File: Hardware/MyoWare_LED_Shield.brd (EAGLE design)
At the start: 52.3 x 21.6 mm, 21 parts, among them IC1 LM3914V, U1 MCP73831

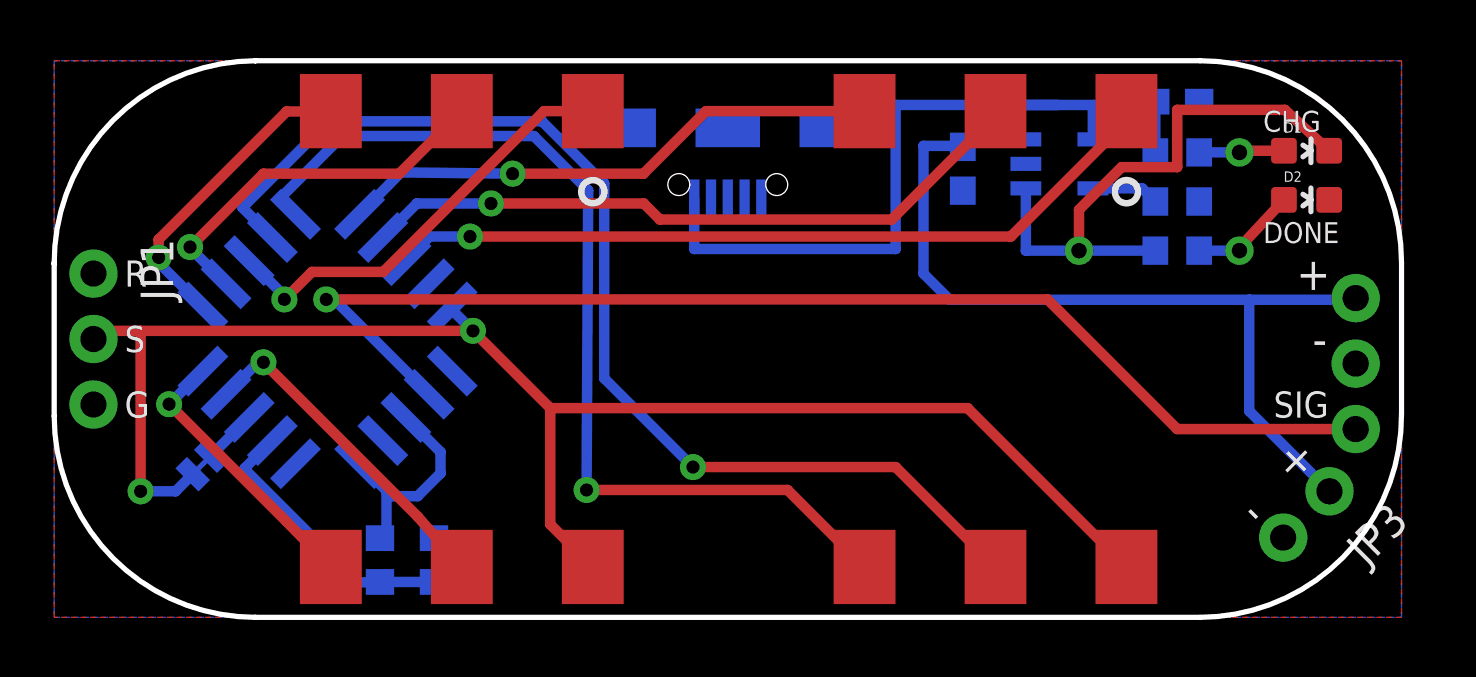
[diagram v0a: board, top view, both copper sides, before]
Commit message: Design rules checked
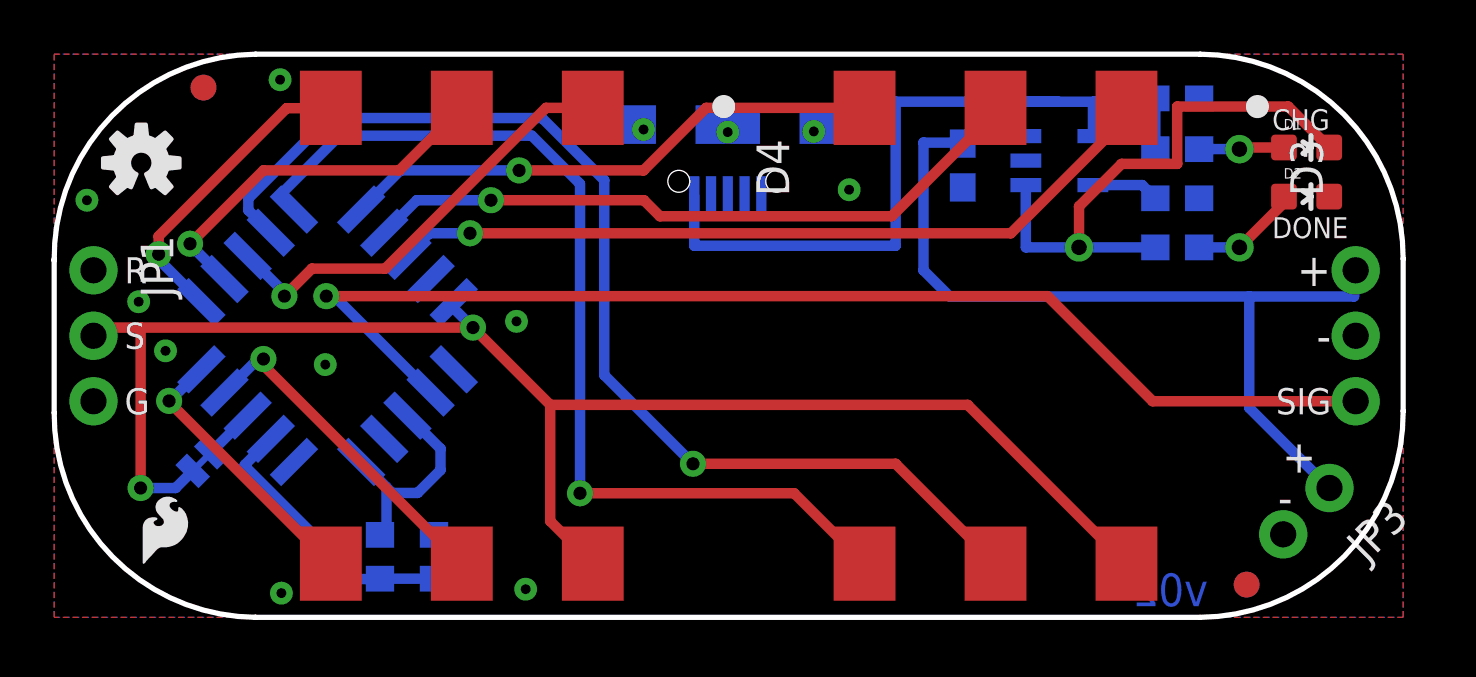
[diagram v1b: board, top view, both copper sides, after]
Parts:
- removed IC1: LM3914V, national-semiconductor:PLCC20S
- removed SJ1: SOLDERJUMPERTRACE, SparkFun:SJ_2S-TRACE
- removed U$1, U$2: SMA-B500, advancer-technologies:LED_BAR_SMD
- added D3, D4: SMA-B500, Testing:LED_BAR_SMD
- added FID1, FID2, FID3, FID4: FIDUCIAL1X2, SparkFun-Aesthetics:FIDUCIAL-1X2
- added LOGO1: SFE_LOGO_FLAME.1_INCH, SparkFun-Aesthetics:SFE_LOGO_FLAME_.1
- added LOGO2: OSHW-LOGOS, SparkFun-Aesthetics:OSHW-LOGO-S
- added MODE: JUMPER-PAD-2-NC_BY_TRACE, SparkFun-Passives:PAD-JUMPER-2-NC_BY_TRACE_YES_SILK
- added U2: LM3914V, Testing:PLCC20S
- JP2: value Power -> Signal
- JP3: value (none) -> LiPo
- R3, R5: device resistor:R0603 -> SparkFun-Resistors:0603-RES
- R4: value 10k -> 10K; device resistor:R0603 -> SparkFun-Resistors:0603-RES
- moved JP2 1.08 mm to (50.5, 13.5)
- moved D2 0.13 mm to (48.6, 16.3)
- moved R3 0.13 mm to (43.6, 18.2)
- moved R5 0.13 mm to (43.6, 14.4)
- moved JP3 0.13 mm to (49.5, 5.02)
- moved R1 0.13 mm to (12.6, 2.35)
- moved R2 0.13 mm to (14.7, 2.35)
- moved U$6 0.13 mm to (26.1, 2.35)
- moved C1 0.13 mm to (43.6, 20.1)
- moved C2 0.13 mm to (35.2, 17.5)
- moved D1 0.13 mm to (48.6, 18.2)
- moved JP1 0.13 mm to (1.52, 13.5)
- moved JP4 0.13 mm to (26.1, 19.1)
- moved R4 0.13 mm to (43.6, 16.3)
- moved U$9 0.13 mm to (4.89, 17.7)
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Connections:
- net N$7 renamed VBUS
- net GND: now also U2.2, U2.4; no longer IC1.2, IC1.4
- net N$1: now also D3.1, U2.1; no longer IC1.1, U$1.1
- net N$11: now also D4.2, U2.15; no longer IC1.15, U$2.2
- net N$12: now also D4.3, U2.14; no longer IC1.14, U$2.3
- net N$13: now also D4.4, U2.13; no longer IC1.13, U$2.4
- net N$14: now also D4.5, U2.12; no longer IC1.12, U$2.5
- net N$19: now also U2.10; no longer IC1.10
- net N$2: now also D3.2, U2.20; no longer IC1.20, U$1.2
- net N$20: now also U2.6, U2.8; no longer IC1.6, IC1.8
- net N$3: now also D3.5, U2.17; no longer IC1.17, U$1.5
- net N$4: now also D3.3, U2.19; no longer IC1.19, U$1.3
- net N$5: now also D4.1, U2.16; no longer IC1.16, U$2.1
- net N$6: now also MODE.1, U2.11; no longer IC1.11, SJ1.1
- net N$8: now also D3.4, U2.18; no longer IC1.18, U$1.4
- net SHLD_PWR: now also D3.6, D4.6, MODE.2, U2.3; no longer IC1.3, SJ1.2, U$1.6, U$2.6
- net SIG: now also U2.5; no longer IC1.5
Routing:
- net +VS: track 35.2 -> 36.1 mm
- net N$3: track 44.1 -> 43.6 mm
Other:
- board size 52.3 x 21.6 mm -> 52.3 x 21.8 mm
- board text added: "ALL UNITS IN INCHES"
- board text added: "LED SHIELD"
- board text added: "MODE"
- board text added: "v02"
